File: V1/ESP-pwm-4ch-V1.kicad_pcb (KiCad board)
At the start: 2 copper layers, 103 x 67.8 mm, 37 parts, among them J1 12VDC, J2 OUT1, J3 OUT2, J4 OUT3, J5 OUT4, Q1 IRLB8721PBF, Q2 IRLB8721PBF, Q3 IRLB8721PBF, Q4 IRLB8721PBF, U1 L78M05, U2 WeMos_D1_mini, U3 Olimex_ESP32-POE, U4 IR4427, U5 IR4427

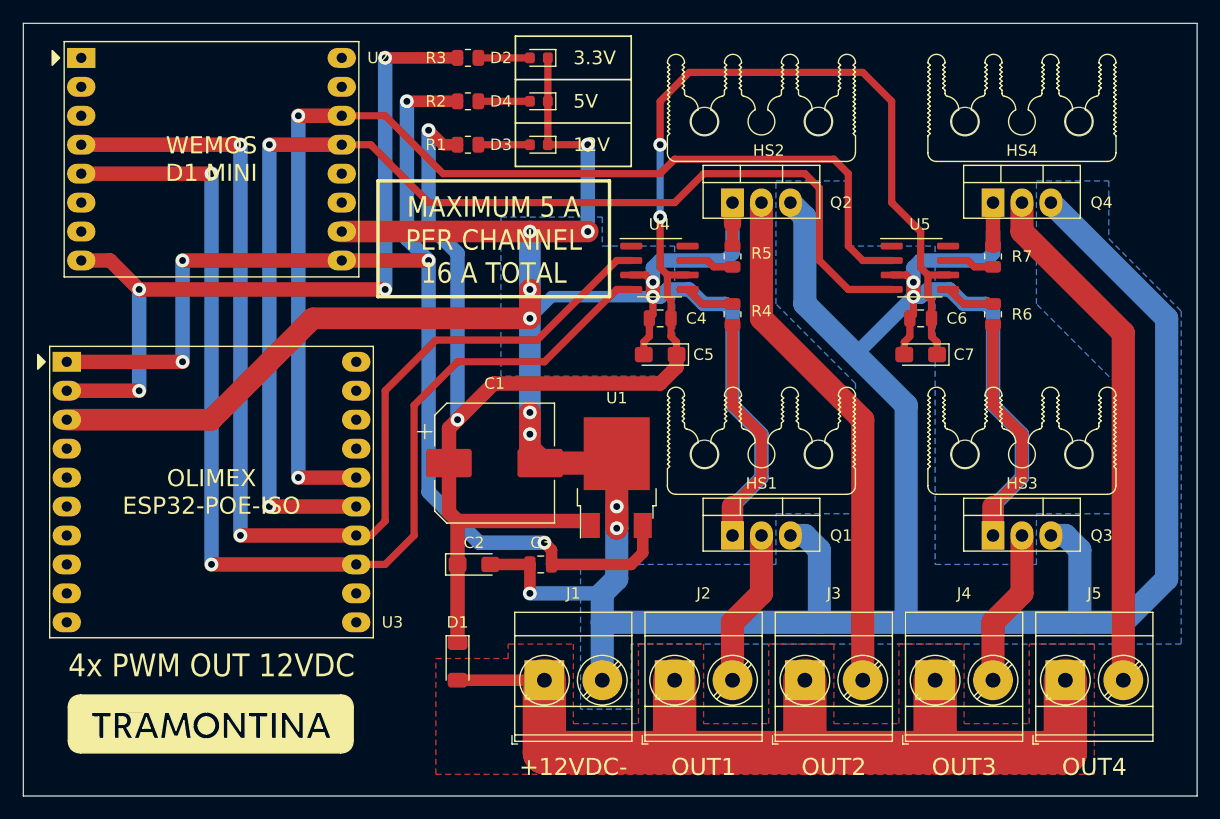
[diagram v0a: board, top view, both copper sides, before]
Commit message: PCB tweaks
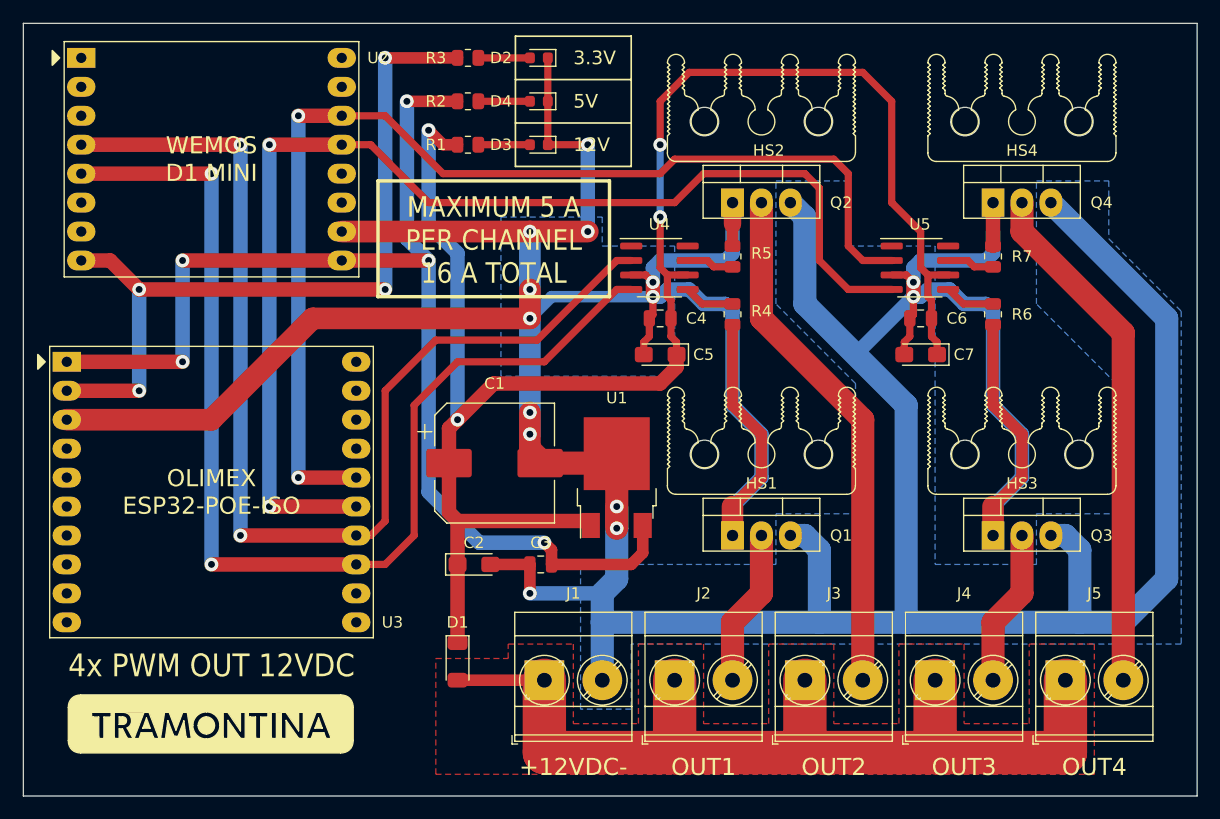
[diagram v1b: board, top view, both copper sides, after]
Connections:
- U2 pad 1: Net-(U2-Pad1) -> unconnected-(U2-Pad1)
- U2 pad 11: Net-(U2-Pad11) -> unconnected-(U2-Pad11)
- U2 pad 12: Net-(U2-Pad12) -> unconnected-(U2-Pad12)
- U2 pad 15: Net-(U2-Pad15) -> unconnected-(U2-Pad15)
- U2 pad 16: Net-(U2-Pad16) -> unconnected-(U2-Pad16)
- U2 pad 2: Net-(U2-Pad2) -> unconnected-(U2-Pad2)
- U2 pad 3: Net-(U2-Pad3) -> unconnected-(U2-Pad3)
- U2 pad 6: Net-(U2-Pad6) -> unconnected-(U2-Pad6)
- U2 pad 7: Net-(U2-Pad7) -> unconnected-(U2-Pad7)
- U3 pad 10: Net-(U3-Pad10) -> unconnected-(U3-Pad10)
- U3 pad 11: Net-(U3-Pad11) -> unconnected-(U3-Pad11)
- U3 pad 12: Net-(U3-Pad12) -> unconnected-(U3-Pad12)
- U3 pad 17: Net-(U3-Pad17) -> unconnected-(U3-Pad17)
- U3 pad 18: Net-(U3-Pad18) -> unconnected-(U3-Pad18)
- U3 pad 19: Net-(U3-Pad19) -> unconnected-(U3-Pad19)
- U3 pad 20: Net-(U3-Pad20) -> unconnected-(U3-Pad20)
- U3 pad 4: Net-(U3-Pad4) -> unconnected-(U3-Pad4)
- U3 pad 5: Net-(U3-Pad5) -> unconnected-(U3-Pad5)
- U3 pad 6: Net-(U3-Pad6) -> unconnected-(U3-Pad6)
- U3 pad 7: Net-(U3-Pad7) -> unconnected-(U3-Pad7)
- U3 pad 8: Net-(U3-Pad8) -> unconnected-(U3-Pad8)
- U3 pad 9: Net-(U3-Pad9) -> unconnected-(U3-Pad9)
- U4 pad 1: Net-(U4-Pad1) -> unconnected-(U4-Pad1)
- U4 pad 8: Net-(U4-Pad8) -> unconnected-(U4-Pad8)
- U5 pad 1: Net-(U5-Pad1) -> unconnected-(U5-Pad1)
- U5 pad 8: Net-(U5-Pad8) -> unconnected-(U5-Pad8)
